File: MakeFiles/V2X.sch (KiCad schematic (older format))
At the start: 0 parts

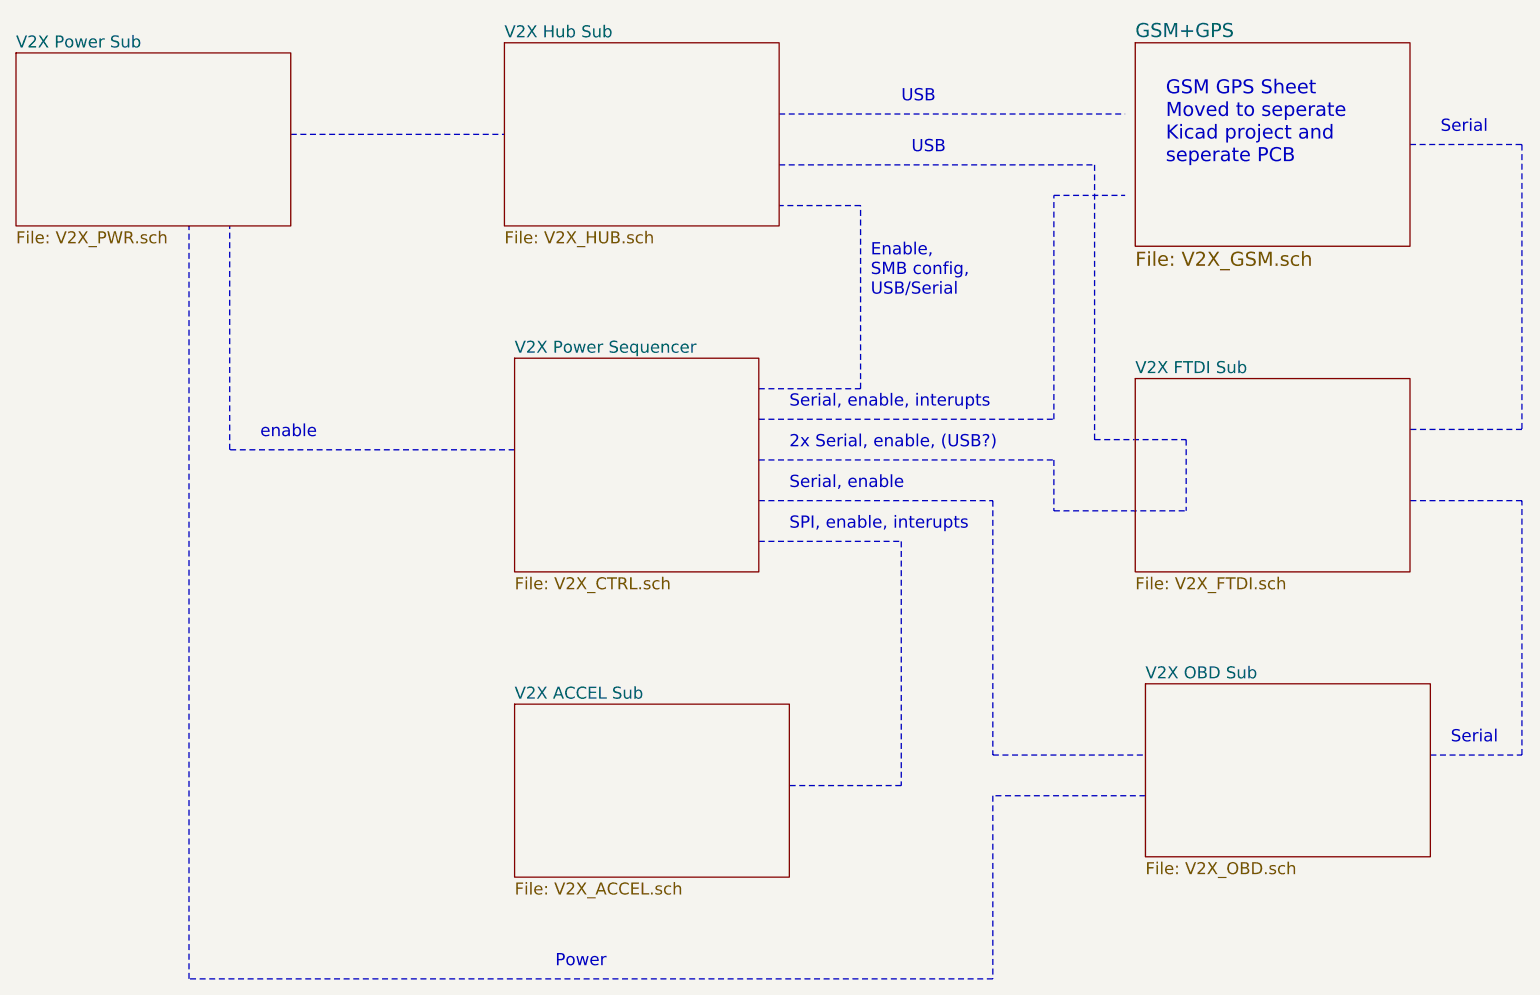
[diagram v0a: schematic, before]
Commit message: 53851 Import of V2X R2.0
capture from legacy repo
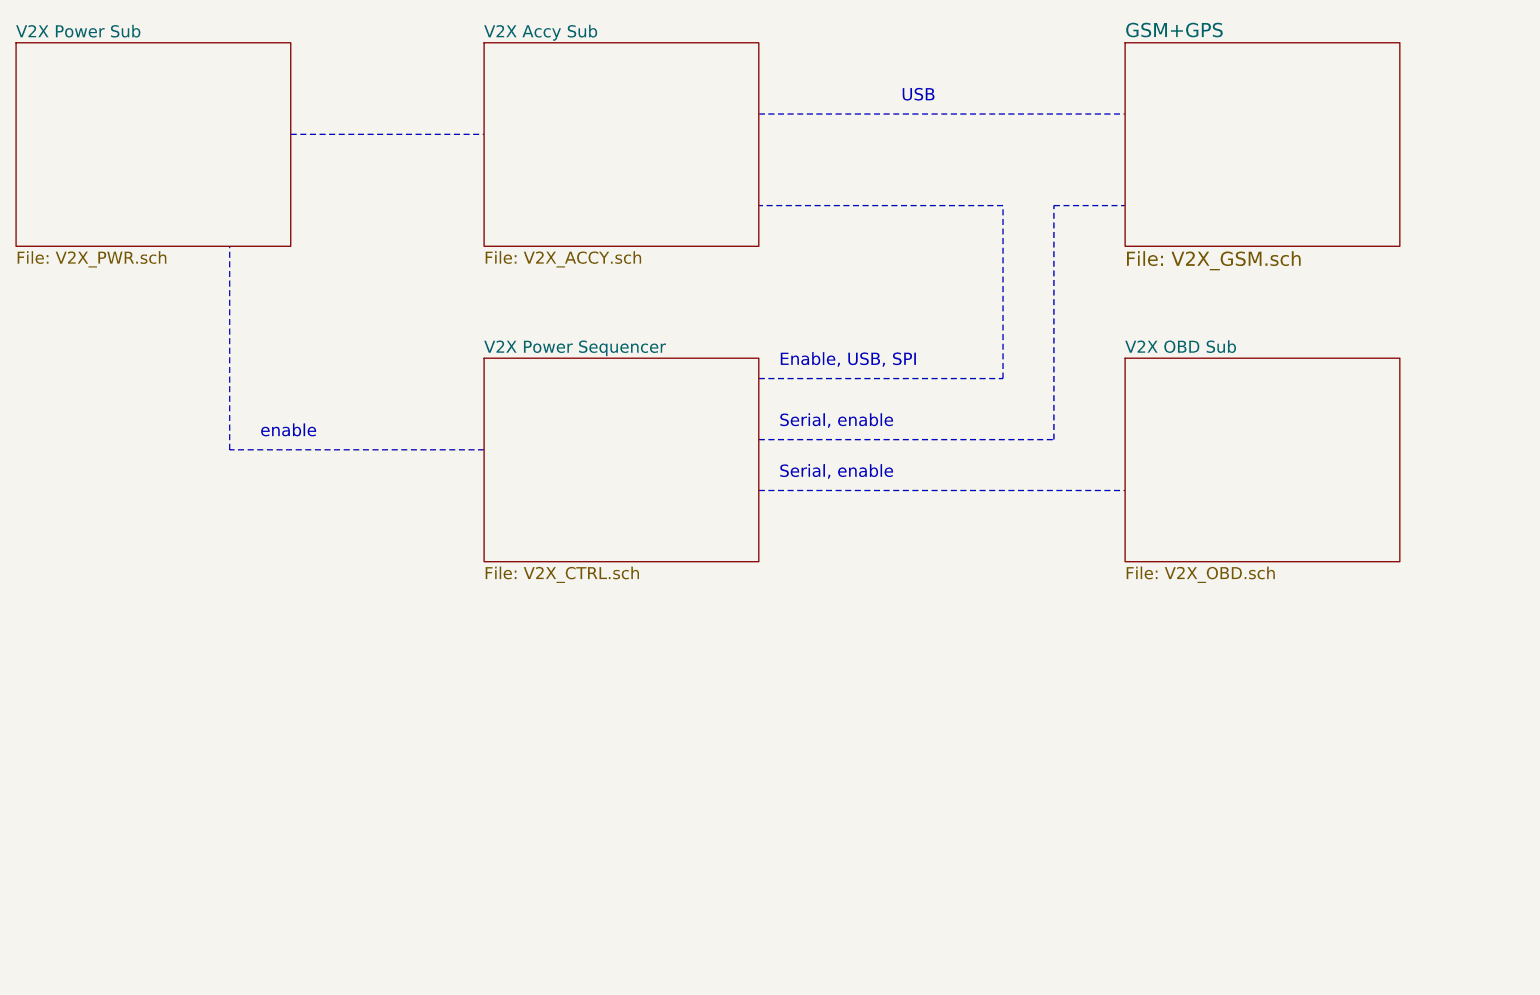
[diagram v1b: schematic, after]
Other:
- note added: "Enable, USB, SPI"
- note removed: "2x Serial, enable, (USB?)"
- note removed: "Enable, \nSMB config,\nUSB/Serial"
- note removed: "GSM GPS Sheet\nMoved to seperate\nKicad project and \nseperate PCB"
- note removed: "Power"
- note removed: "SPI, enable, interupts"
- note removed: "Serial"
- note removed: "Serial, enable, interupts"
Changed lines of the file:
@@
 $Descr USLetter 11000 8500
 encoding utf-8
-Sheet 1 8
+Sheet 1 6
 Title "V2X - Open source RVI over SMS daughter card"
 Date "2015-07-17"
@@
 $EndDescr
 $Sheet
-S 7450 2750 1350 950
-U 55AB1D0F
-F0 "V2X FTDI Sub" 59
-F1 "V2X_FTDI.sch" 59
-$EndSheet
-$Sheet
-S 7500 4250 1400 850
+S 7400 2650 1350 1000
 U 55AB3ADF
 F0 "V2X OBD Sub" 59
@@
 $EndSheet
 $Sheet
-S 1950 1150 1350 850
+S 1950 1100 1350 1000
 U 55AB3850
 F0 "V2X Power Sub" 59
@@
 $EndSheet
 $Sheet
-S 4400 4350 1350 850
-U 55AFC3B8
-F0 "V2X ACCEL Sub" 59
-F1 "V2X_ACCEL.sch" 59
+S 4250 1100 1350 1000
+U 55F8B2F2
+F0 "V2X Accy Sub" 59
+F1 "V2X_ACCY.sch" 59
 $EndSheet
 $Sheet
-S 4350 1100 1350 900
-U 55F8B2F2
-F0 "V2X Hub Sub" 59
-F1 "V2X_HUB.sch" 59
-$EndSheet
-$Sheet
-S 4400 2650 1200 1050
+S 4250 2650 1350 1000
 U 55F91B74
 F0 "V2X Power Sequencer" 59
@@
 $EndSheet
 Wire Notes Line
-	4400 3100 3000 3100
+	4250 3100 3000 3100
 Wire Notes Line
-	3000 3100 3000 2000
+	3000 3100 3000 2100
 Wire Notes Line
-	3300 1550 4350 1550
+	3300 1550 4250 1550
 Wire Notes Line
-	5700 1450 7400 1450
+	5600 1450 7400 1450
 Wire Notes Line
-	5600 3350 6750 3350
+	5600 3300 7400 3300
 Wire Notes Line
-	6750 3350 6750 4600
+	5600 2750 6800 2750
 Wire Notes Line
-	6750 4600 7500 4600
+	6800 2750 6800 1900
 Wire Notes Line
-	5600 3550 6300 3550
-Wire Notes Line
-	6300 3550 6300 4750
-Wire Notes Line
-	6300 4750 5750 4750
-Wire Notes Line
-	5600 3150 7050 3150
-Wire Notes Line
-	7050 3150 7050 3400
-Wire Notes Line
-	7050 3400 7700 3400
-Wire Notes Line
-	5700 1700 7250 1700
-Wire Notes Line
-	7250 1700 7250 3050
-Wire Notes Line
-	7250 3050 7700 3050
-Wire Notes Line
-	5600 2800 6100 2800
-Wire Notes Line
-	6100 2800 6100 1900
-Wire Notes Line
-	6100 1900 5700 1900
-Text Notes 6150 2350 0    60   ~ 0
-Enable, \nSMB config,\nUSB/Serial
+	6800 1900 5600 1900
+Text Notes 5700 2700 0    60   ~ 0
+Enable, USB, SPI
 Text Notes 6300 1400 0    60   ~ 0
 USB
-Text Notes 6350 1650 0    60   ~ 0
-USB
-Text Notes 8950 1550 0    60   ~ 0
-Serial
-Text Notes 9000 4550 0    60   ~ 0
-Serial
-Text Notes 5750 2900 0    60   ~ 0
-Serial, enable, interupts
-Text Notes 5750 3300 0    60   ~ 0
+Text Notes 5700 3000 0    60   ~ 0
 Serial, enable
-Text Notes 5750 3500 0    60   ~ 0
-SPI, enable, interupts
+Text Notes 5700 3250 0    60   ~ 0
+Serial, enable
 Text Notes 3150 3050 0    60   ~ 0
 enable
 Wire Notes Line
-	7500 4800 6750 4800
+	5600 3050 7050 3050
 Wire Notes Line
-	6750 4800 6750 5700
+	7050 3050 7050 1900
 Wire Notes Line
-	6750 5700 2800 5700
-Wire Notes Line
-	2800 5700 2800 2000
-Text Notes 4600 5650 0    60   ~ 0
-Power
-Text Notes 5750 3100 0    60   ~ 0
-2x Serial, enable, (USB?)
-Wire Notes Line
-	5600 2950 7050 2950
-Wire Notes Line
-	7050 2950 7050 1850
-Wire Notes Line
-	7050 1850 7400 1850
-Text Notes 7600 1700 0    69   ~ 0
-GSM GPS Sheet\nMoved to seperate\nKicad project and \nseperate PCB
-Wire Notes Line
-	7700 3050 7700 3400
-Wire Notes Line
-	8900 4600 9350 4600
-Wire Notes Line
-	9350 4600 9350 3350
-Wire Notes Line
-	9350 3350 8800 3350
-Wire Notes Line
-	8800 1600 9350 1600
-Wire Notes Line
-	9350 1600 9350 3000
-Wire Notes Line
-	9350 3000 8800 3000
+	7050 1900 7400 1900
 $Sheet
-S 7450 1100 1350 1000
+S 7400 1100 1350 1000
 U 562004BB
 F0 "GSM+GPS" 69
